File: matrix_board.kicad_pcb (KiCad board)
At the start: 2 copper layers, 49.5 x 27.3 mm, 8 parts, among them J1 MATRIX_CONNECTOR, M1 PWR_LED, M2 LED, U1 ATmega328P-AU

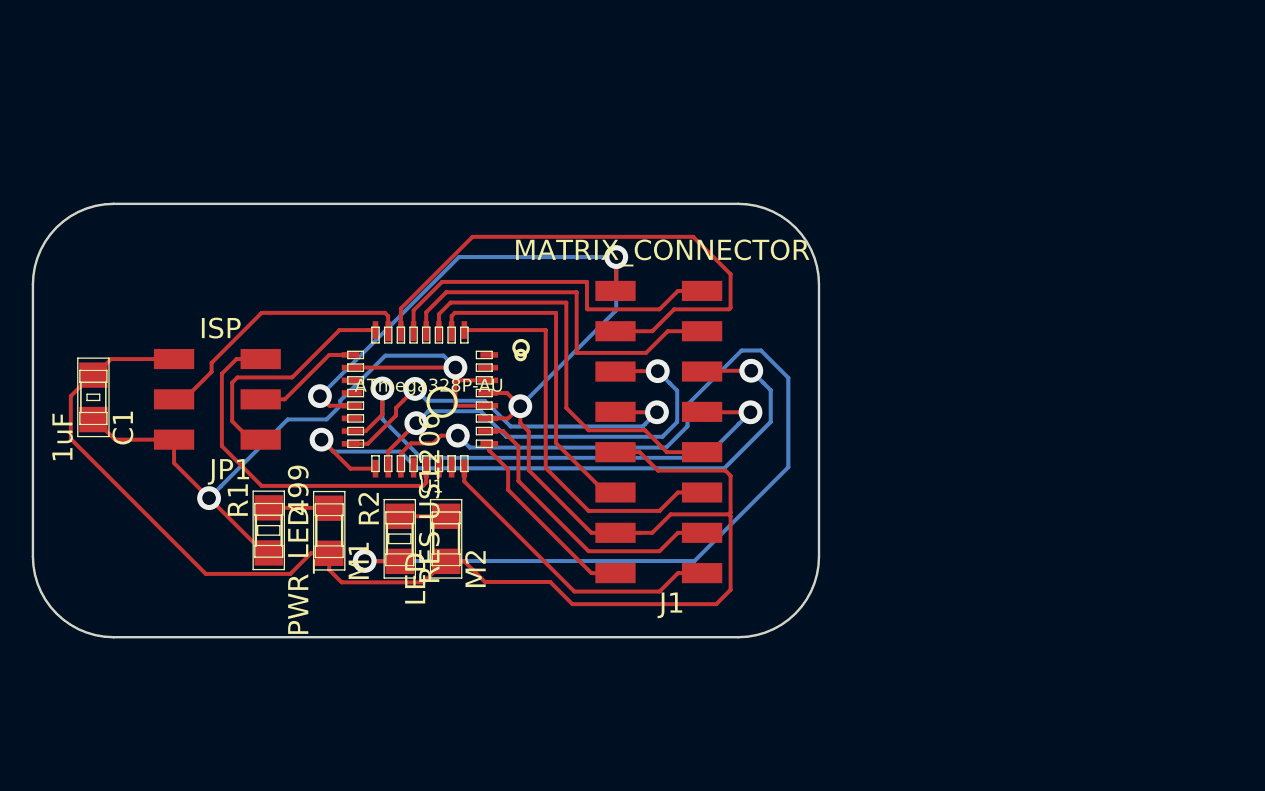
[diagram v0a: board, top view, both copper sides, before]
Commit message: added new board design. hope it works
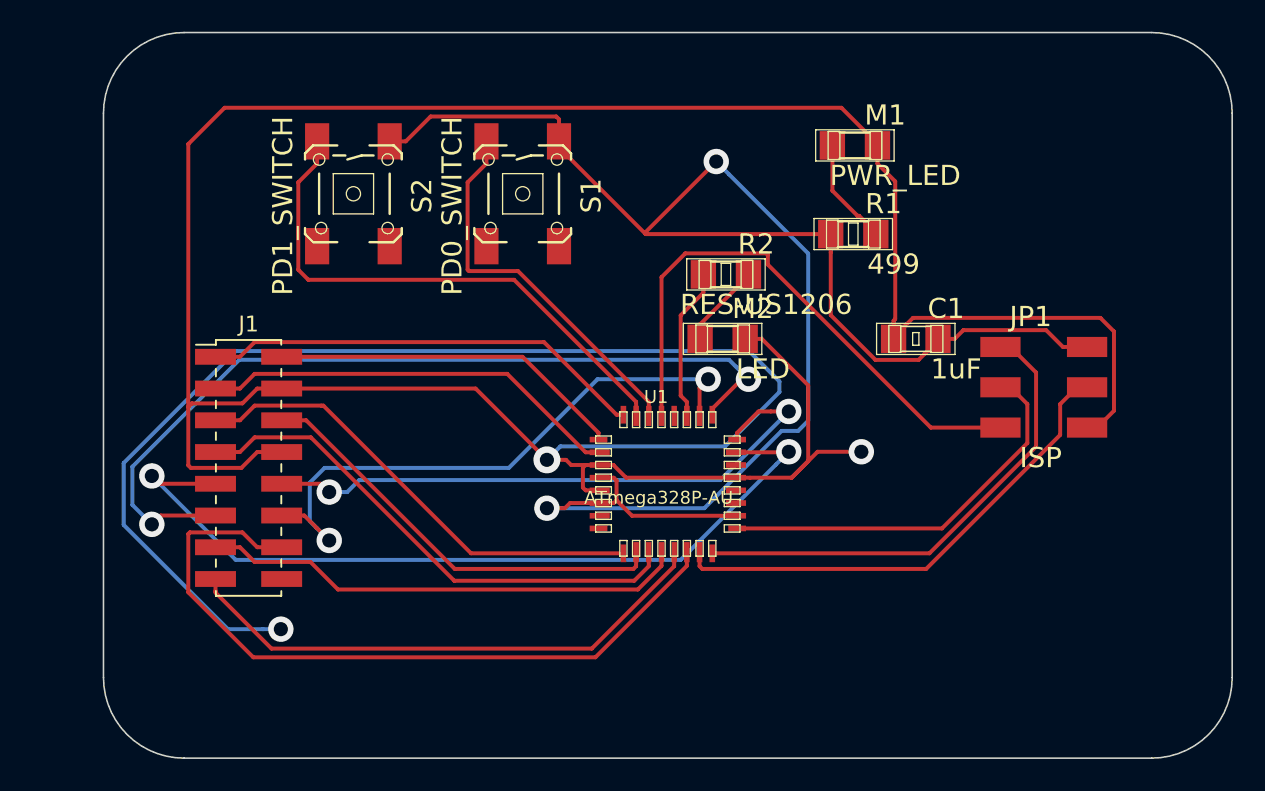
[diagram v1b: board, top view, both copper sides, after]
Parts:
- added S1: PD0_SWITCH, fab:fab-6MM_SWITCH, F.Cu at (148.3, 55.9)
- added S2: PD1_SWITCH, fab:fab-6MM_SWITCH, F.Cu at (137.7, 55.9)
- C1: footprint kicad_fab:fab-C1206 -> fab:fab-C1206
- J1: footprint fab:fab-2X16SMD -> Connector_PinHeader_2.00mm:PinHeader_2x08_P2.00mm_Vertical_SMD
- JP1: footprint kicad_fab:fab-2X03SMD -> fab:fab-2X03SMD
- M1, M2: footprint kicad_fab:fab-LED1206 -> fab:fab-LED1206
- R1, R2: footprint kicad_fab:fab-R1206 -> fab:fab-R1206
- moved C1 51.9 mm to (173.1, 65.0), turned to 0 degrees
- moved JP1 51.7 mm to (181.0, 68.1), turned to 0 degrees
- moved R1 41.3 mm to (169.2, 58.4), turned to 0 degrees
- moved M1 41.1 mm to (169.3, 52.8), turned to 0 degrees
- moved R2 26.5 mm to (161.1, 61.0), turned to 0 degrees
- moved J1 26.4 mm to (131.1, 73.2), turned to 0 degrees
- moved M2 21.5 mm to (160.9, 65.0), turned to 0 degrees
- moved U1 16.5 mm to (157.5, 74.2), turned to 0 degrees
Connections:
- U1 pad 30: Net-(U1-Pad30) -> PD0
- U1 pad 31: Net-(U1-Pad31) -> PD1
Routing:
- net GROUND: track 136.8 -> 245.3 mm
- net VCC: track 48.2 -> 115.1 mm
- net TEST: track 67.1 -> 9.67 mm, vias 2 -> 0
- net PD1: track 0.00 -> 34.2 mm
- net PD0: track 0.00 -> 24.3 mm
- net A: track 34.4 -> 52.7 mm
- net SCK: track 7.46 -> 25.1 mm
- net MISO: track 15.1 -> 30.8 mm
- net MOSI: track 17.1 -> 31.3 mm
- net B: track 25.0 -> 38.5 mm
- net RESET: track 22.9 -> 35.6 mm
- net C: track 41.3 -> 53.9 mm
- net OE: track 22.4 -> 34.3 mm
- net LAT: track 35.0 -> 46.4 mm
- net D: track 27.7 -> 38.1 mm
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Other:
- board size 49.5 x 27.3 mm -> 71.1 x 45.7 mm
- net class Default: clearance 0.4 -> 0.3; via_dia 0.8 -> 1.6; via_drill 0.4 -> 0.89
- rule pad_to_mask_clearance: 0.051 -> 0
- rule trace_clearance: 0.4 -> 0.3
